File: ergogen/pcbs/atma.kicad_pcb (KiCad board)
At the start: 2 copper layers, 99.8 x 100 mm, 24 parts

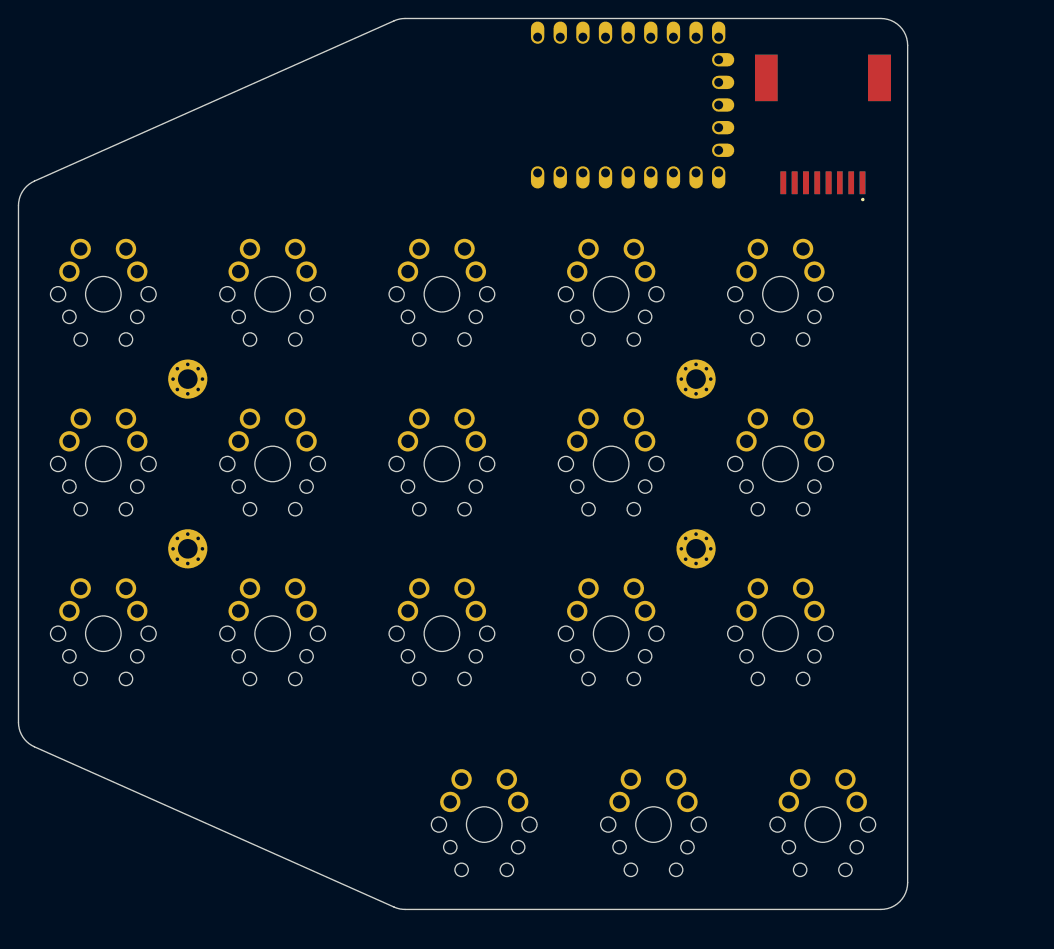
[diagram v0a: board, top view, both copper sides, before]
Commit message: atma v0.2.0 (#2)
* atma v0.2.0
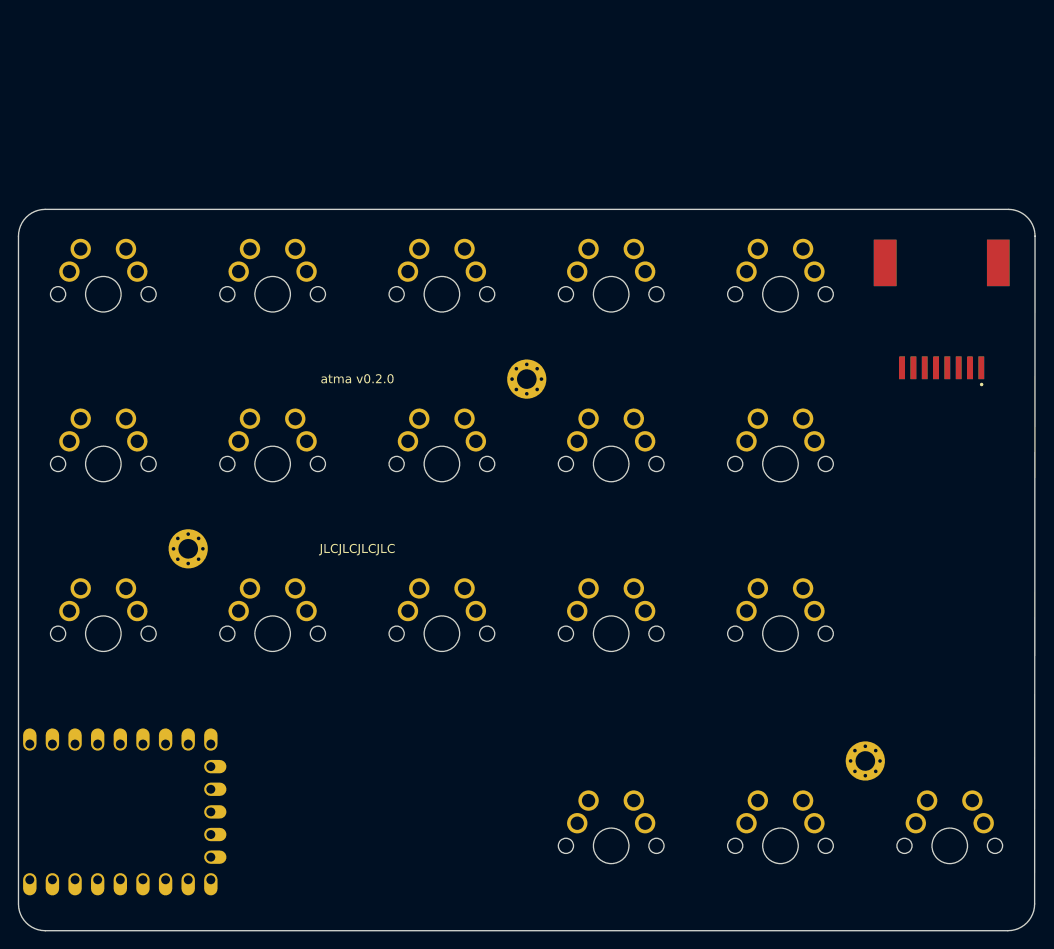
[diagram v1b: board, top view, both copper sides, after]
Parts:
- removed _6: , MountingHole_2.2mm_M2_Pad_Via
- moved ? 97.7 mm to (154.3, 172.4)
- moved _5 46.9 mm to (237.9, 166.7)
- moved _4 42.6 mm to (199.9, 123.8)
- moved ? 24.7 mm to (246.5, 121.7)
- moved _3 19.1 mm to (161.9, 142.9)
- moved S16 14.4 mm to (209.4, 176.2)
- moved S17 14.4 mm to (228.4, 176.2)
- moved S18 14.4 mm to (247.4, 176.2)
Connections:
- ? pad 1: matrix_pinky_bottom -> matrix_pinky_top
- ? pad 10: GP9 -> matrix_index_bottom
- ? pad 11: matrix_middle_top -> matrix_index_home
- ? pad 12: matrix_inner_bottom -> matrix_index_top
- ? pad 13: matrix_inner_home -> GP12
- ? pad 14: matrix_inner_top -> GP13
- ? pad 15: matrix_index_top -> matrix_inner_top
- ? pad 16: matrix_index_home -> matrix_inner_home
- ? pad 17: matrix_index_bottom -> matrix_inner_bottom
- ? pad 18: thumbfan_far_home -> thumbfan_near_home
- ? pad 20: thumbfan_near_home -> thumbfan_far_home
- ? pad 3: matrix_pinky_top -> matrix_pinky_bottom
- ? pad 4: matrix_ring_top -> matrix_ring_bottom
- ? pad 6: matrix_ring_bottom -> matrix_ring_top
- ? pad 7: matrix_middle_bottom -> matrix_middle_top
- ? pad 9: GP8 -> matrix_middle_bottom
- ? pad 3: GP8 -> GP13
- ? pad 4: GP8 -> GP13
- ? pad 5: GP9 -> GP12
- ? pad 6: GP9 -> GP12
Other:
- board size 99.8 x 100 mm -> 114.1 x 81 mm
- board text added: "JLCJLCJLCJLC"
- board text added: "atma v0.2.0"
